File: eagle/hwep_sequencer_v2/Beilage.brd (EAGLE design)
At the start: 251.5 x 99.1 mm, 119 parts, among them X1 ESP32-DEVKIT-C

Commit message: reroute brd complete
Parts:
- X1: value ESP32-DEVKIT-C -> ESP32CLIP2122; device modul_GruS:ESP32-DEVKIT-C -> modul_GruS:ESP32-DEVKIT-C-CLIP
- moved R1 80.1 mm to (153.7, 67.3), flipped to the bottom, turned to 90 degrees
- moved H2 79.6 mm to (168.9, 73.7), turned to 90 degrees
- moved R7 79.0 mm to (168.9, 76.2), turned to 180 degrees
- moved C4 78.6 mm to (220.3, 67.3), turned to 0 degrees
- moved X1 73.3 mm to (176.5, 74.9), turned to 270 degrees
- moved X4 65.9 mm to (222.2, 71.1), flipped to the bottom, turned to 270 degrees
- moved R12 63.8 mm to (207.0, 78.7), turned to 90 degrees
- moved R13 63.3 mm to (204.5, 78.7), turned to 90 degrees
- moved R14 63.0 mm to (201.9, 78.7), turned to 90 degrees
- moved C3 62.5 mm to (168.9, 53.3), flipped to the bottom, turned to 270 degrees
- moved D3 60.8 mm to (163.8, 62.2), flipped to the bottom
- moved X3 52.4 mm to (218.4, 71.1)
- moved R15 51.6 mm to (207.0, 53.3), turned to 180 degrees
- moved R23 41.9 mm to (172.2, 67.3), flipped to the bottom
- moved R19 41.2 mm to (172.2, 62.2), flipped to the bottom
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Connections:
- removed net N$71: H11.4, H8.2
- removed net N$8: D9.4, H3.4
- new net DI: D9.4, H11.4
- new net DO: H14.2, H3.4
- net AGND: now also X1.22
- net VREF: now also X1.21
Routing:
- net +3V3: track 809.7 -> 678.4 mm, vias 5 -> 6
- net 23S08_!CS: track 127.7 -> 55.1 mm
- net 7SEG_CH: track 77.7 -> 6.23 mm, vias 1 -> 0
- net 7SEG_CZ: track 67.4 -> 5.70 mm, vias 2 -> 0
- net 7SEG_CE: track 62.2 -> 5.96 mm, vias 2 -> 0
- net SCK: track 143.2 -> 89.6 mm, vias 3 -> 2
- net STP_CS: track 79.3 -> 31.1 mm, vias 2 -> 1
- net MOSI: track 85.8 -> 38.3 mm, vias 1 -> 2
- net INT_23S08: track 63.9 -> 19.3 mm
- net N$7: track 26.6 -> 68.8 mm, vias 0 -> 1
- net N$8: track 32.5 -> 0.00 mm
- net MISO: track 94.4 -> 65.7 mm
- net PL_DIN: track 3.79 -> 30.6 mm
- net AGND: track 276.2 -> 302.2 mm, vias 1 -> 2
- net ADC088S052_!CS: track 70.9 -> 93.1 mm
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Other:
- board size 251.5 x 99.1 mm -> 227.3 x 82.5 mm

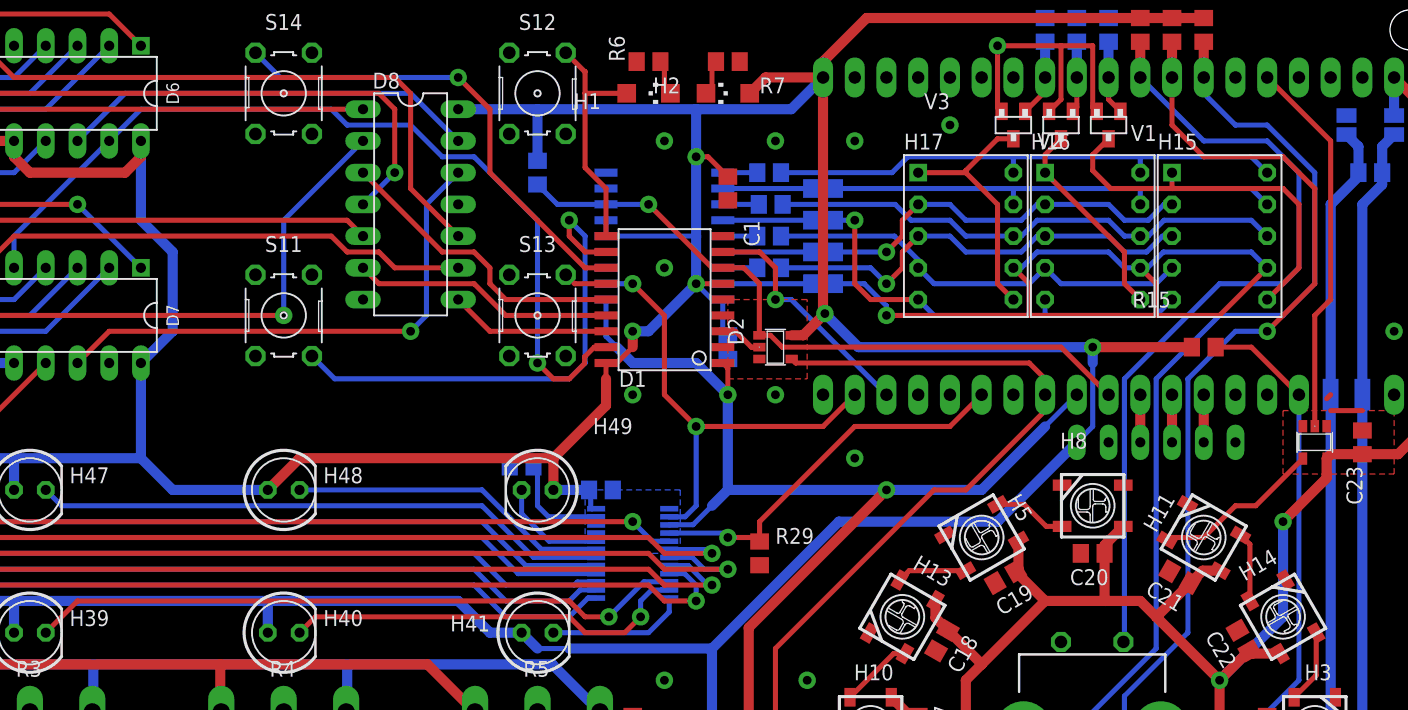
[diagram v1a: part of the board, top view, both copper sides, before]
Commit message: optimized brd and 3d model
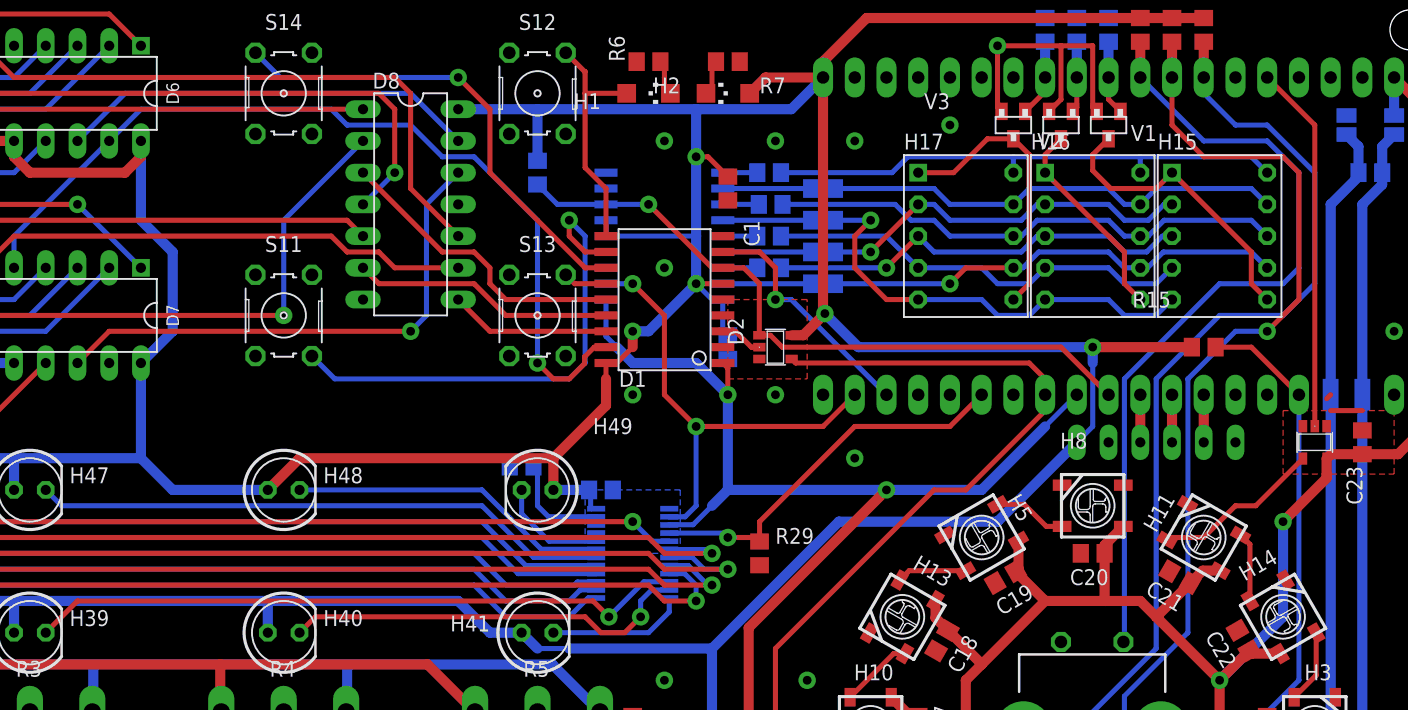
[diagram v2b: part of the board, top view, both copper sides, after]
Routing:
- net N$7: track 68.8 -> 37.2 mm
- net N$55: track 30.6 -> 23.9 mm
- net N$65: track 20.6 -> 22.7 mm
- net N$33: track 36.3 -> 34.5 mm
- net EC11_B: track 79.1 -> 78.1 mm
- net PL_DIN: track 30.6 -> 29.5 mm
- net N$56: track 34.9 -> 35.8 mm
- net N$35: track 31.4 -> 30.7 mm
